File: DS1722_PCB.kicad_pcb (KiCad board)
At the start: 2 copper layers, 13 parts, among them J1 Conn_01x08_Male, J2 Conn_01x08_Male, U1 DS1722

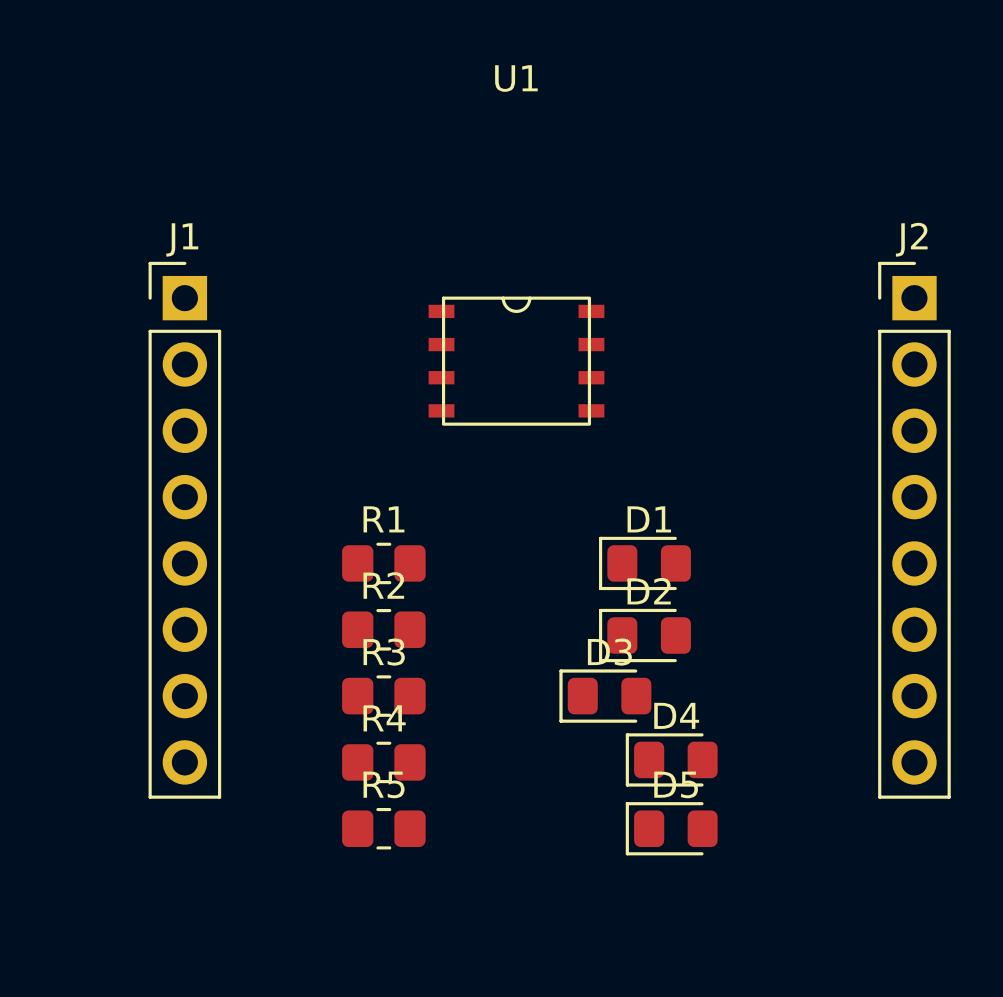
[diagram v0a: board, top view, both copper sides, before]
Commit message: Finished layout
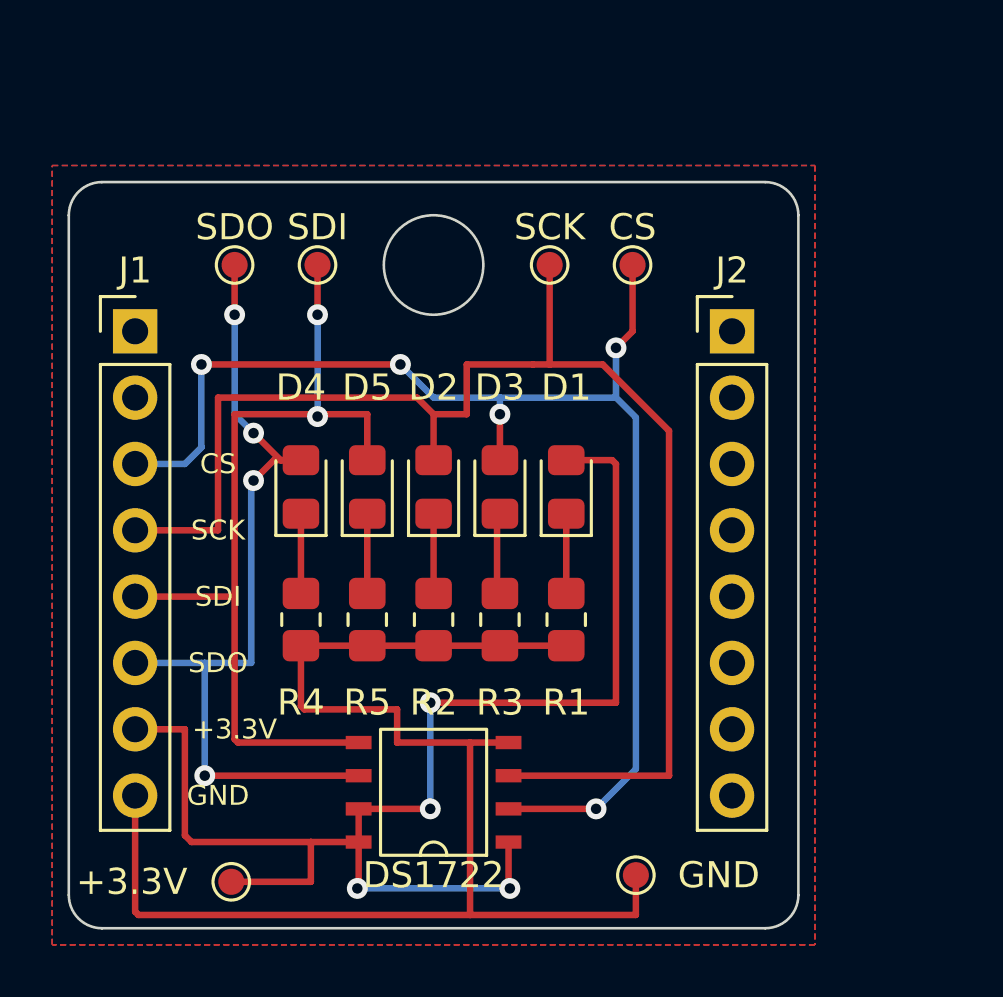
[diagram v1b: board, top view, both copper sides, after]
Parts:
- added +3.3V: TestPoint_Pad_D1.0mm, TestPoint:TestPoint_Pad_D1.0mm, F.Cu at (113.5, 90.9)
- added CS: TestPoint_Pad_D1.0mm, TestPoint:TestPoint_Pad_D1.0mm, F.Cu at (128.9, 67.3)
- added GND: TestPoint_Pad_D1.0mm, TestPoint:TestPoint_Pad_D1.0mm, F.Cu at (129.0, 90.7)
- added SCK: TestPoint_Pad_D1.0mm, TestPoint:TestPoint_Pad_D1.0mm, F.Cu at (125.7, 67.3)
- added SDI: TestPoint_Pad_D1.0mm, TestPoint:TestPoint_Pad_D1.0mm, F.Cu at (116.8, 67.3)
- added SDO: TestPoint_Pad_D1.0mm, TestPoint:TestPoint_Pad_D1.0mm, F.Cu at (113.7, 67.3)
- moved D4 17.8 mm to (116.2, 75.8), turned to 90 degrees
- moved D5 17.6 mm to (118.7, 75.8), turned to 90 degrees
- moved U1 16.6 mm to (121.3, 87.4), turned to 180 degrees
- moved D2 10.0 mm to (121.3, 75.8), turned to 90 degrees
- moved D3 9.04 mm to (123.8, 75.8), turned to 90 degrees
- moved R5 8.04 mm to (118.7, 80.9), turned to -90 degrees
- moved R1 7.31 mm to (126.4, 80.9), turned to -90 degrees
- moved J2 7.10 mm to (132.7, 69.8)
- moved R4 6.32 mm to (116.2, 80.9), turned to -90 degrees
- moved R3 5.32 mm to (123.8, 80.9), turned to -90 degrees
- moved D1 4.32 mm to (126.4, 75.8), turned to 90 degrees
- moved J1 2.29 mm to (109.9, 69.8)
- moved R2 1.94 mm to (121.3, 80.9), turned to -90 degrees
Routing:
- net /SCK: track 0.00 -> 53.7 mm
- net GND: track 0.00 -> 53.5 mm
- net /+3.3V: track 0.00 -> 53.0 mm, vias 0 -> 4
- net /CS: track 0.00 -> 50.2 mm, vias 0 -> 5
- net /MISO: track 0.00 -> 33.7 mm, vias 0 -> 2
- net /MOSI: track 0.00 -> 32.8 mm, vias 0 -> 4
- net Net-(D3-Pad1): track 0.00 -> 3.10 mm
- net Net-(D5-Pad1): track 0.00 -> 3.06 mm
- net Net-(D4-Pad1): track 0.00 -> 3.06 mm
- net Net-(D2-Pad1): track 0.00 -> 3.06 mm
- net Net-(D1-Pad1): track 0.00 -> 3.06 mm
- added copper zone on B.Cu, net GND
- added copper zone on F.Cu, net GND
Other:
- board outline added: 27.9 x 28.6 mm
- board text added: "+3.3V"
- board text added: "CS"
- board text added: "DS1722 Board v.1 E155 Fall '24 Ellie Sundheim"
- board text added: "GND"
- board text added: "SCK"
- board text added: "SDI"
- board text added: "SDO"
